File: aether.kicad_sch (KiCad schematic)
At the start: 41 parts, among them Q1 NPN, Q2 CSD17575Q3, Q3 CSD17575Q3, Q4 CSD17575Q3, Q5 CSD17575Q3, SW1 TDD01H0SB1R, U1 USBLC6-2SC6

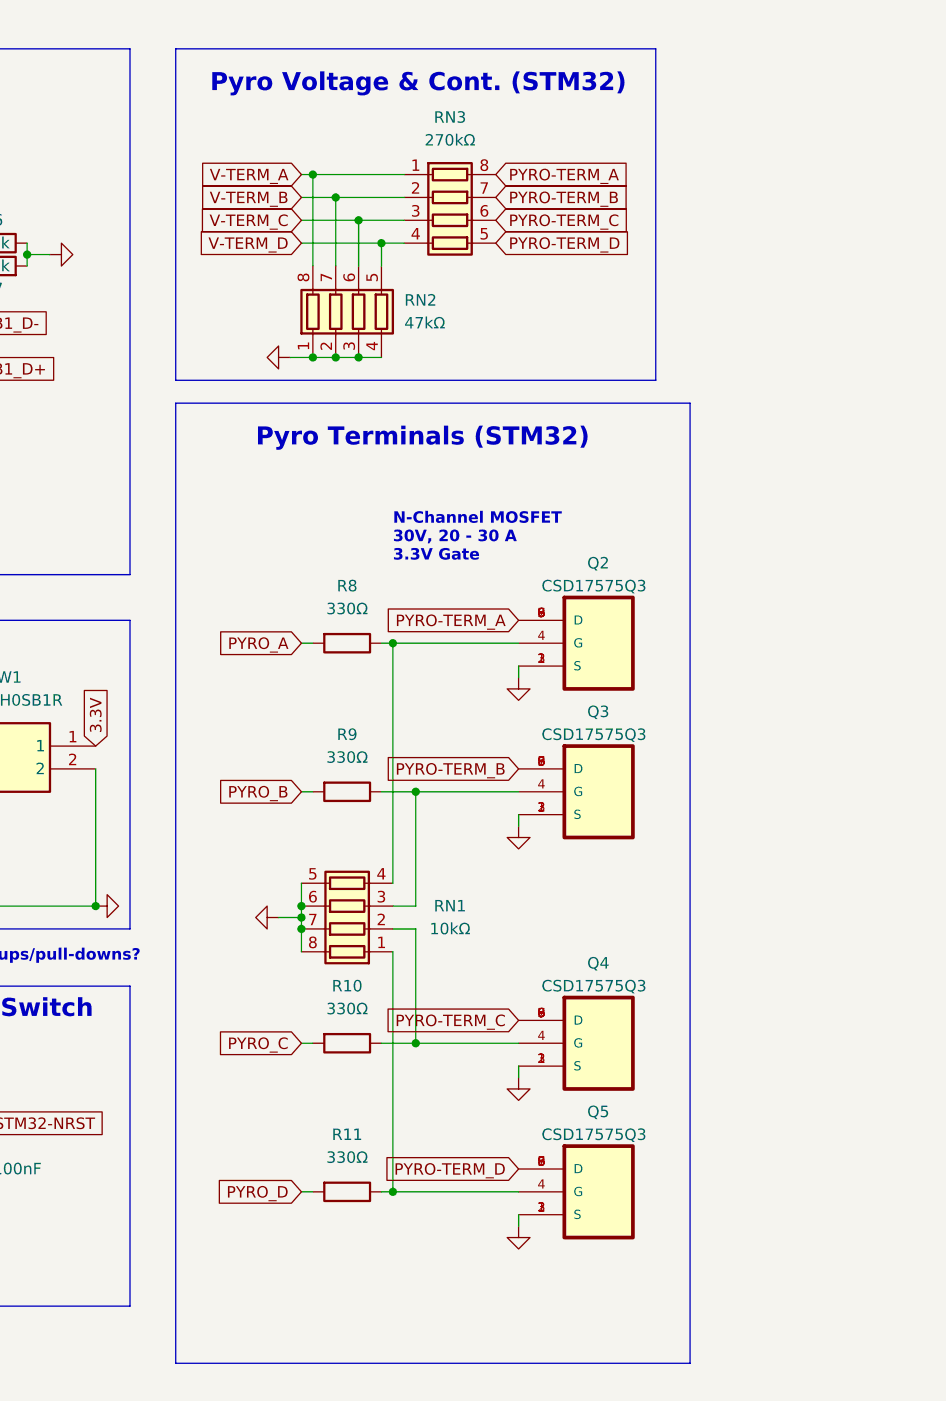
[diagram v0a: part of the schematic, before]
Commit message: more routing
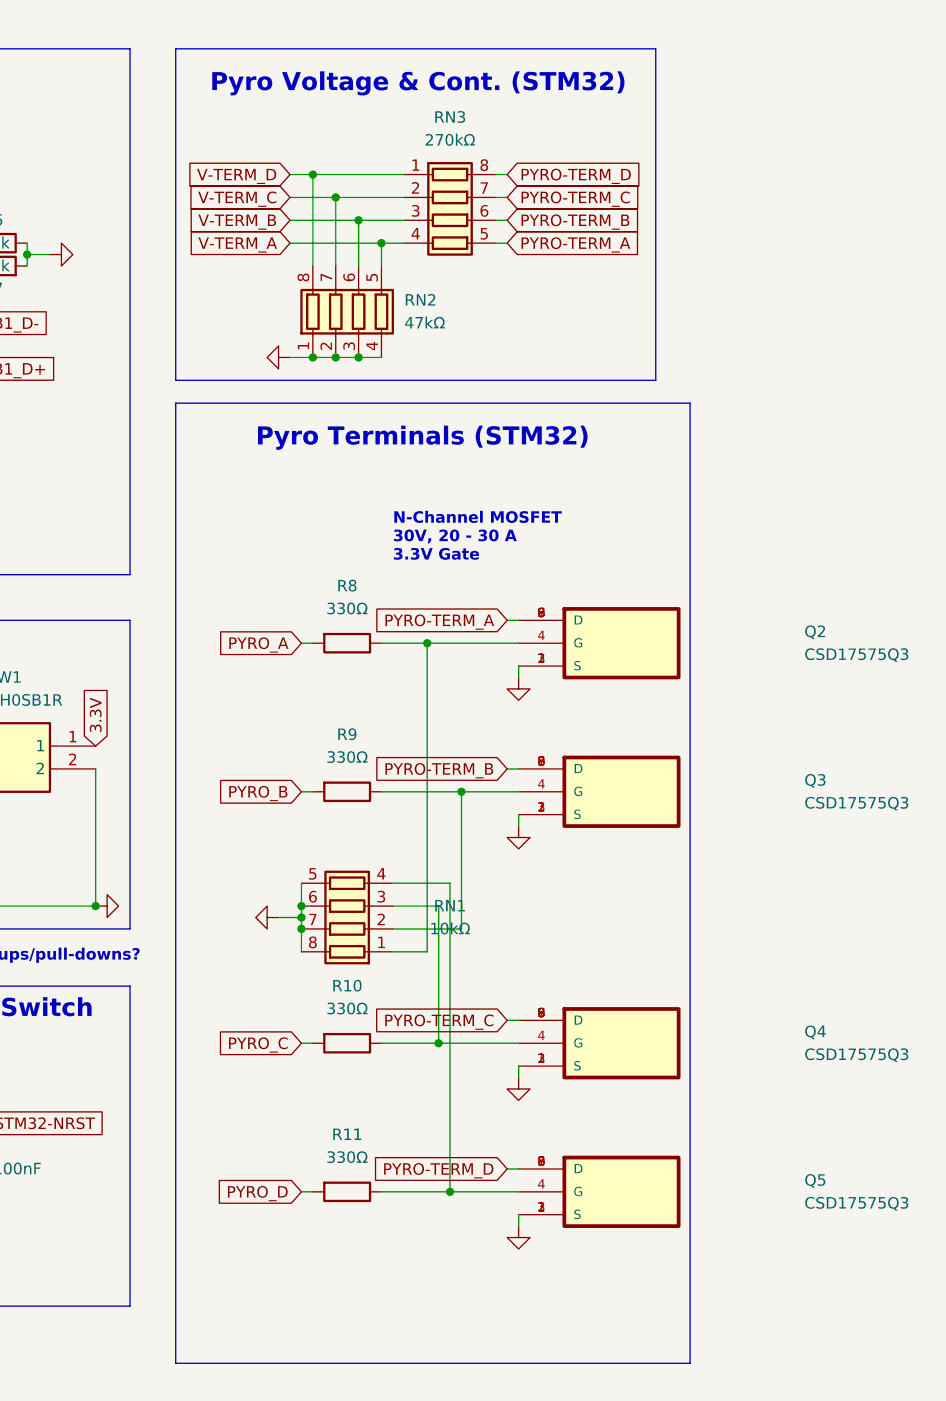
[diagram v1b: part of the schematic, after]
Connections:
- net PYRO-TERM_A: now also RN3.5 (R4.2); no longer RN3.8 (R1.2)
- net PYRO-TERM_B: now also RN3.6 (R3.2); no longer RN3.7 (R2.2)
- net PYRO-TERM_C: now also RN3.7 (R2.2); no longer RN3.6 (R3.2)
- net PYRO-TERM_D: now also RN3.8 (R1.2); no longer RN3.5 (R4.2)
- net V-TERM_A: now also RN2.5 (R4.2), RN3.4 (R4.1); no longer RN2.8 (R1.2), RN3.1 (R1.1)
- net V-TERM_B: now also RN2.6 (R3.2), RN3.3 (R3.1); no longer RN2.7 (R2.2), RN3.2 (R2.1)
- net V-TERM_C: now also RN2.7 (R2.2), RN3.2 (R2.1); no longer RN2.6 (R3.2), RN3.3 (R3.1)
- net V-TERM_D: now also RN2.8 (R1.2), RN3.1 (R1.1); no longer RN2.5 (R4.2), RN3.4 (R4.1)
- net at Q5.4 (G), R11.1: now also RN1.4 (R4.1); no longer RN1.1 (R1.1)
- net at Q4.4 (G), R10.1: now also RN1.3 (R3.1); no longer RN1.2 (R2.1)
- net at Q3.4 (G), R9.1: now also RN1.2 (R2.1); no longer RN1.3 (R3.1)
- net at Q2.4 (G), R8.1: now also RN1.1 (R1.1); no longer RN1.4 (R4.1)
